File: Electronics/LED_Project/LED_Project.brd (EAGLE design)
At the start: 30.5 x 59.4 mm, 17 parts, among them IC1 7805T

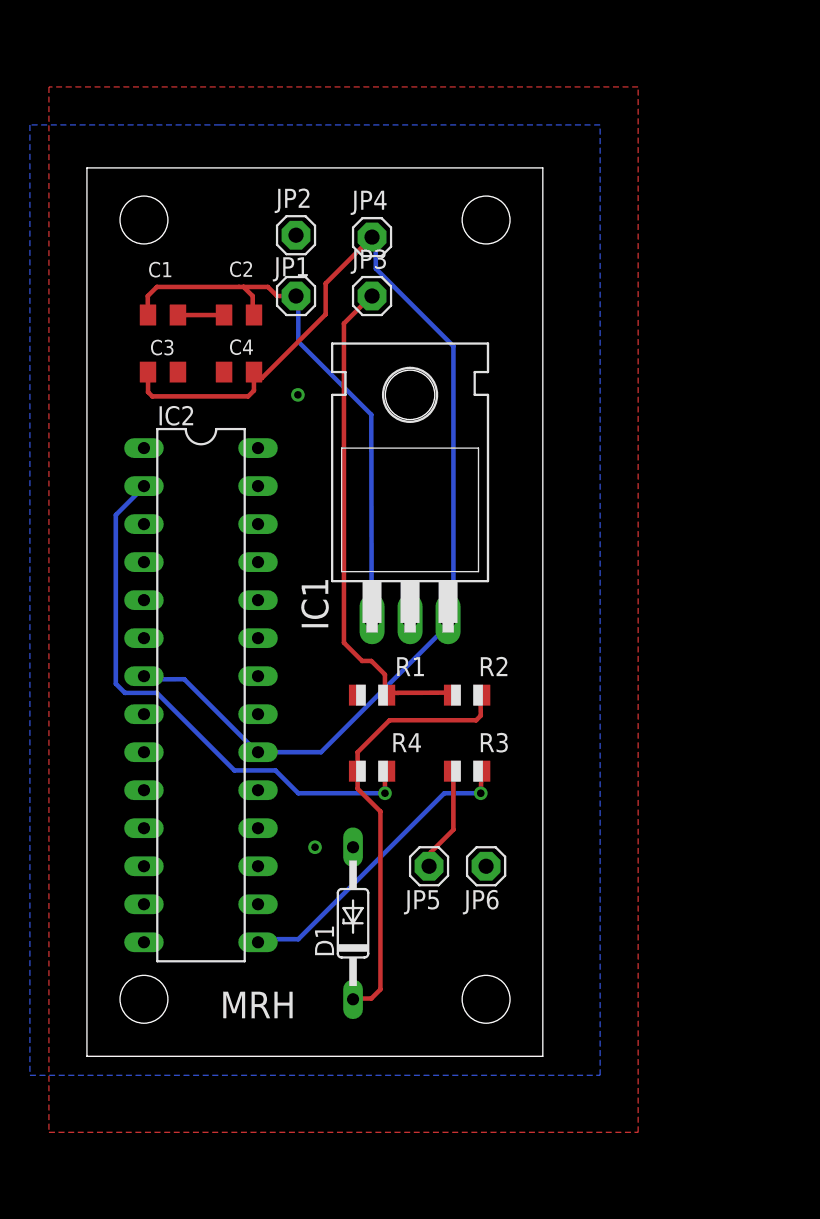
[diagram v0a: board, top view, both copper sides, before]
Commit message: replacecd ECAD files
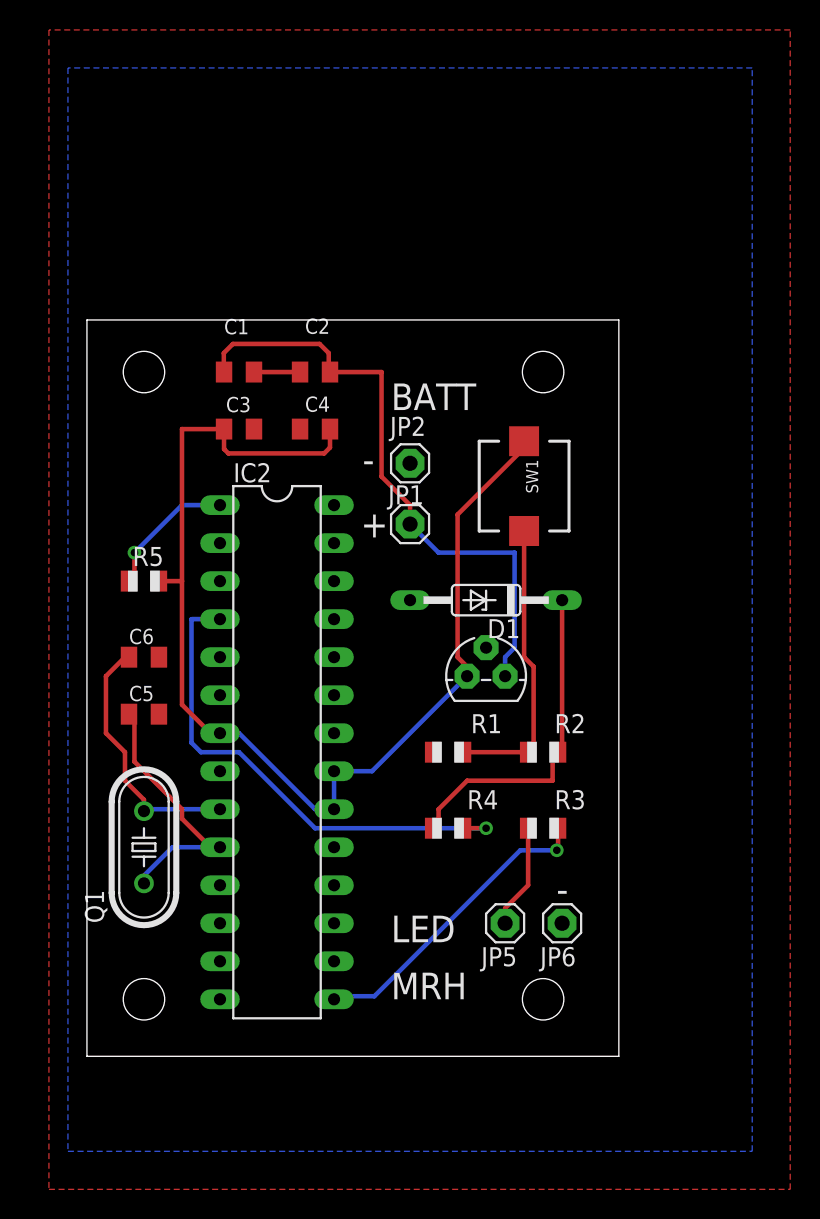
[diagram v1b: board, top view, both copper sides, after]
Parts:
- removed IC1: 7805T, linear:TO220H
- removed JP3, JP4: (no value), adafruit:1X01
- added C5, C6: 22p, adafruit:C0805K
- added IC3: 7805L, adafruit:TO92
- added Q1: (no value), adafruit:HC49/S
- added R5: 10k, adafruit:R0805
- added SW1: (no value), adafruit:PUSHBUTTON_SMD_SJ
- moved D1 23.3 mm to (26.7, 30.5), turned to 180 degrees
- moved JP1 17.0 mm to (21.6, 35.6)
- moved JP2 17.0 mm to (21.6, 39.6)
- moved C1 6.35 mm to (10.2, 45.7)
- moved C2 6.35 mm to (15.2, 45.7)
- moved C3 6.35 mm to (10.2, 41.9)
- moved C4 6.35 mm to (15.2, 41.9)
- moved R3 6.35 mm to (30.5, 15.2)
- moved JP5 6.35 mm to (27.9, 8.89)
- moved R2 6.35 mm to (30.5, 20.3)
- moved IC2 6.35 mm to (12.7, 20.3)
- moved R4 6.35 mm to (24.1, 15.2)
- moved JP6 6.35 mm to (31.8, 8.89)
- moved R1 6.35 mm to (24.1, 20.3)
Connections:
- new net N$10: C5.1, IC2.10, Q1.1
- new net N$12: IC2.1, R5.1
- new net N$4: C6.1, IC2.9, Q1.2
- net +5V: now also IC2.21, IC3.1, R5.2, SW1.P$2; no longer IC1.3, JP4.1
- net GND: now also C5.2, C6.2, IC3.2; no longer IC1.2
- net N$1: now also IC3.3; no longer IC1.1
- net N$2: now also SW1.P$1; no longer JP3.1
- net N$3: now also IC2.4; no longer IC2.2
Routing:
- net N$10: track 0.00 -> 18.4 mm
- net N$4: track 0.00 -> 17.3 mm
- net N$2: track 33.5 -> 19.8 mm
- net N$12: track 0.00 -> 9.30 mm, vias 0 -> 1
- net N$5: track 29.3 -> 22.7 mm
- net N$1: track 37.9 -> 41.1 mm
- net N$3: track 36.5 -> 33.8 mm
- net +5V: track 78.3 -> 77.6 mm
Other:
- board size 30.5 x 59.4 mm -> 35.5 x 49.2 mm
- board text added: "+"
- board text added: "-"
- board text added: "BATT"
- board text added: "LED"
